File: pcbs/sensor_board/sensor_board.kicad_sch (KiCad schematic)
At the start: 41 parts, among them J1 1.5mm, J2 2.5mm, J3 2.5mm, J4 1.5 mm, J5 RJ45, J6 Conn_01x06, Q1 220mA / 50V, Q2 220mA / 50V, Q3 220mA / 50V, U1 8-28V in / 5V 5W out, U2 I2C Dual Rheostat 100kOhm 8-b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, U3 8x GPIO, U4 4x PWM

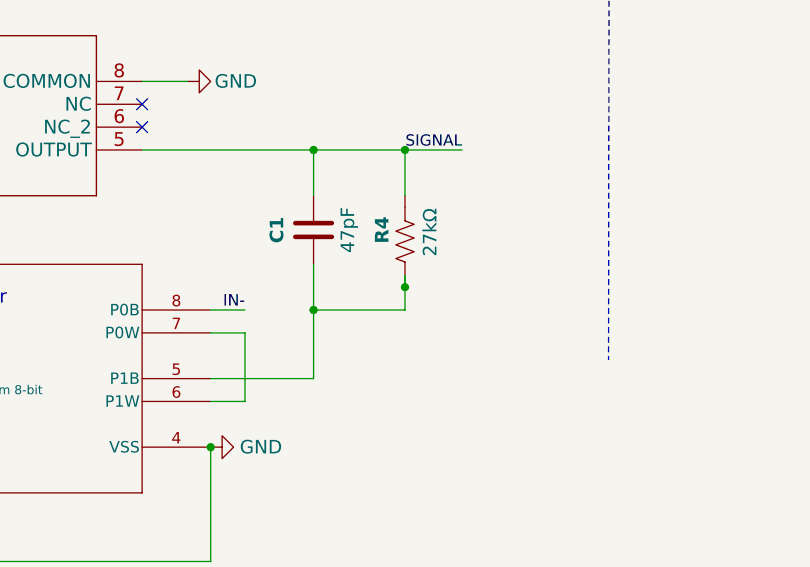
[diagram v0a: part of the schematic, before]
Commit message: sensor board version 1.1
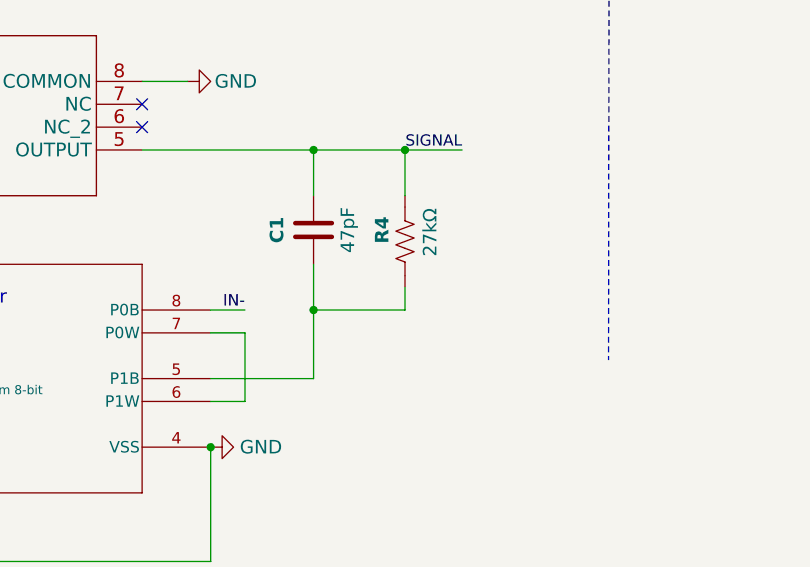
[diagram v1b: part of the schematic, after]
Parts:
- D1: JLCPCB C125085 -> C125086; JLCPCBURL https://jlcpcb.com/partdetail/LiteOn-LTSTC150KGKT/C125085 -> https://jlcpcb.com/partdetail/LiteOn-LTSTC150KRKT/C125086
- R1: JLCPCB C4410 -> (none); JLCPCBURL https://jlcpcb.com/partdetail/4817-1206W4F1001T5E/C4410 -> (none)
- R11, R12, R13, R14: JLCPCB C17902 -> (none); JLCPCBURL https://jlcpcb.com/partdetail/18590-1206W4F1002T5E/C17902 -> (none)
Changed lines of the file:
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@@
 	)
 	(junction
-		(at 251.46 199.39)
-		(diameter 0)
-		(color 0 0 0 0)
-	)
-	(junction
 		(at 350.52 129.54)
 		(diameter 0)
@@
 	(wire
 		(pts
-			(xy 251.46 199.39) (xy 251.46 201.93)
-		)
-		(stroke
-			(width 0)
-			(type default)
-		)
-	)
-	(wire
-		(pts
 			(xy 304.8 52.07) (xy 304.8 50.8)
 		)
@@
 	(wire
 		(pts
-			(xy 251.46 198.12) (xy 251.46 199.39)
+			(xy 251.46 199.39) (xy 251.46 201.93)
 		)
 		(stroke
@@
 			)
 		)
-		(property "JLCPCB" "C4410"
-			(at 312.42 171.45 0)
-			(effects
-				(font
-					(size 1.27 1.27)
-				)
-				(hide yes)
-			)
-		)
-		(property "JLCPCBURL" "https://jlcpcb.com/partdetail/4817-1206W4F1001T5E/C4410"
-			(at 312.42 171.45 0)
-			(effects
-				(font
-					(size 1.27 1.27)
-				)
-				(hide yes)
-			)
-		)
 		(pin "1"
 		)
@@
 			)
 		)
-		(property "JLCPCB" "C125085"
+		(property "JLCPCB" "C125086"
 			(at 58.42 63.5 0)
 			(effects
@@
 			)
 		)
-		(property "JLCPCBURL" "https://jlcpcb.com/partdetail/LiteOn-LTSTC150KGKT/C125085"
+		(property "JLCPCBURL" "https://jlcpcb.com/partdetail/LiteOn-LTSTC150KRKT/C125086"
 			(at 58.42 63.5 0)
 			(effects
@@
 			)
 		)
-		(property "JLCPCB" "C17902"
-			(at 219.71 63.5 0)
-			(effects
-				(font
-					(size 1.27 1.27)
-				)
-				(hide yes)
-			)
-		)
-		(property "JLCPCBURL" "https://jlcpcb.com/partdetail/18590-1206W4F1002T5E/C17902"
-			(at 219.71 63.5 0)
-			(effects
-				(font
-					(size 1.27 1.27)
-				)
-				(hide yes)
-			)
-		)
 		(pin "1"
 		)
@@
 			)
 		)
-		(property "JLCPCB" "C17902"
-			(at 219.71 71.12 0)
-			(effects
-				(font
-					(size 1.27 1.27)
-				)
-				(hide yes)
-			)
-		)
-		(property "JLCPCBURL" "https://jlcpcb.com/partdetail/18590-1206W4F1002T5E/C17902"
-			(at 219.71 71.12 0)
-			(effects
-				(font
-					(size 1.27 1.27)
-				)
-				(hide yes)
-			)
-		)
 		(pin "1"
 		)
@@
 			)
 		)
-		(property "JLCPCB" "C17902"
-			(at 215.9 50.8 0)
-			(effects
-				(font
-					(size 1.27 1.27)
-				)
-				(hide yes)
-			)
-		)
-		(property "JLCPCBURL" "https://jlcpcb.com/partdetail/18590-1206W4F1002T5E/C17902"
-			(at 215.9 50.8 0)
-			(effects
-				(font
-					(size 1.27 1.27)
-				)
-				(hide yes)
-			)
-		)
 		(pin "1"
 		)
@@
 			(at 219.71 78.74 0)
 			(effects
-				(font
-					(size 1.27 1.27)
-				)
-				(hide yes)
-			)
-		)
-		(property "JLCPCB" "C17902"
-			(at 219.71 78.74 0)
-			(effects
-				(font
-					(size 1.27 1.27)
-				)
-				(hide yes)
-			)
-		)
-		(property "JLCPCBURL" "https://jlcpcb.com/partdetail/18590-1206W4F1002T5E/C17902"
-			(at 219.71 78.74 0)
-			(effects
